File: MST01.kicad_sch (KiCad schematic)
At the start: 46 parts, among them J1 AMPSeal-35-verticale-nero, J1 USB_B_Mini, J2 AMPSeal-35-verticale-bianco, J3 Conn_01x04_Pin, J6 Conn_01x05_Pin, M1 Module-power_12and5V-0.2, M3 Module-knock-0.2, M3 Module-vr-discrete-0.5, M4 Module-vr-max9924-0.1, M5 Module-wbo-0.5, M6 Module:mega-mcu100/0.3, M7 Module-can-0.1, P1 Pad, P10 Pad, P2 Pad, P3 Pad, P4 Pad, P5 Pad, P6 Pad, P7 Pad, P8 Pad, P9 Pad, U5 JDY-33

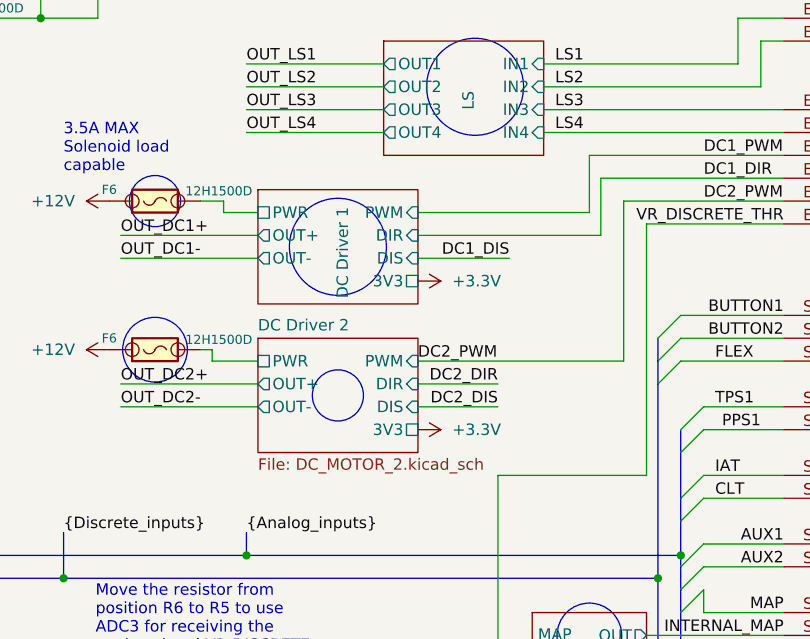
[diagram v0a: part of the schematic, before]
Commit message: Aggiornamento Progetto
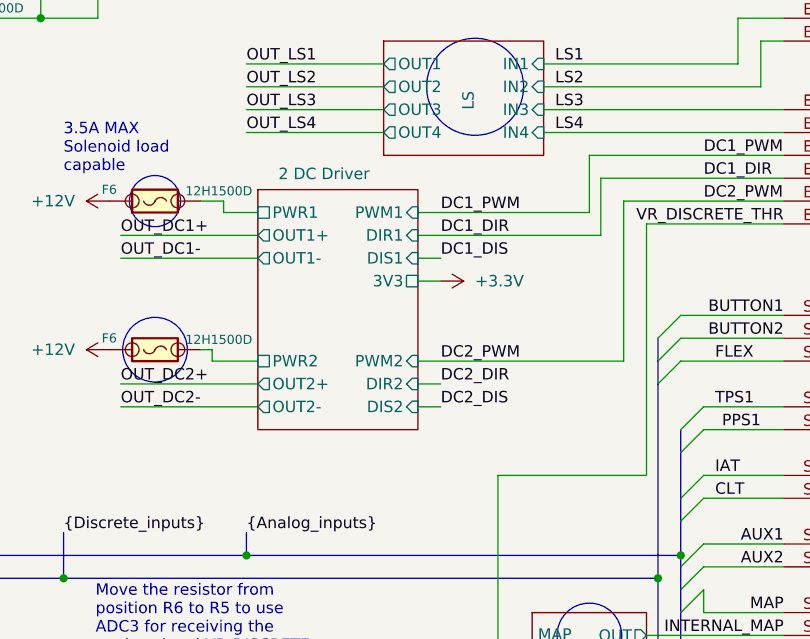
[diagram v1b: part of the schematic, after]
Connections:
- net 2 DC Driver/PWR renamed 2 DC Driver/PWR1
- net DC Driver 2/PWR renamed 2 DC Driver/PWR2
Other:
- sheet DC Driver 1 renamed 2 DC Driver
- removed sheet DC Driver 2
- sheet 2 DC Driver: file DC_MOTOR_1.kicad_sch -> 2_DC_MOTOR.kicad_sch
- sheet 2 DC Driver ports: added DIR1, DIR2, DIS1, DIS2, OUT1+, OUT1-, OUT2+, OUT2-, PWM1, PWM2, PWR1, PWR2; removed DIR, DIS, OUT+, OUT-, PWM, PWR
